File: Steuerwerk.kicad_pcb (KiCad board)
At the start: 2 copper layers, 100 x 160 mm, 115 parts, among them J1 Conn_01x04, J2 Conn_01x02, J3 Conn_01x03, J4 Conn_01x03, J5 Conn_01x02, J6 Conn_01x04, J7 Conn_01x02, J8 Conn_01x04, Q1 Q_PNP_BCE, U1 74LS161, U2 74LS138, U3 74LS138, U4 74240, U5 74LS374, U6 74LS374, U7 74541, U8 74541

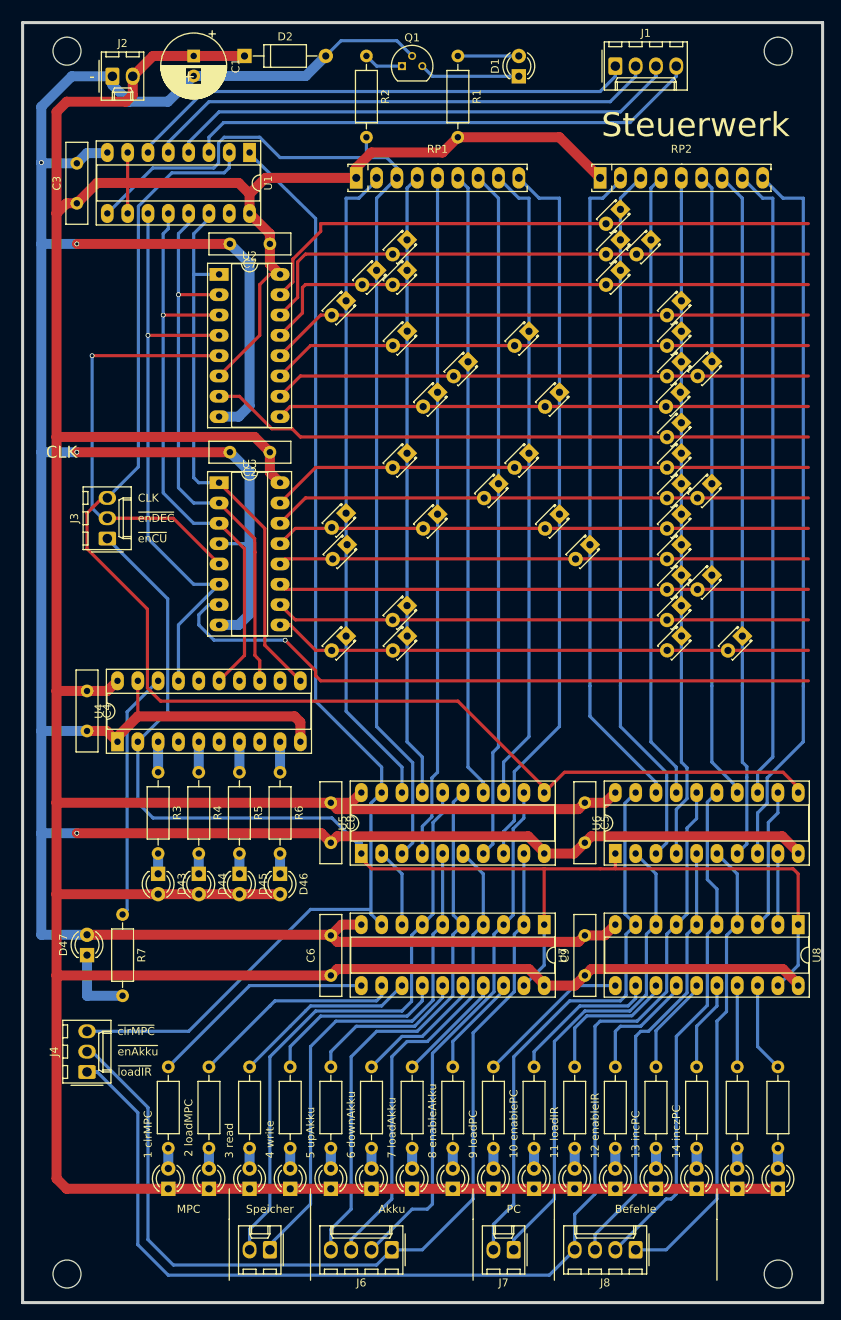
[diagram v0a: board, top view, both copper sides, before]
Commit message: viele Kleinigkeiten
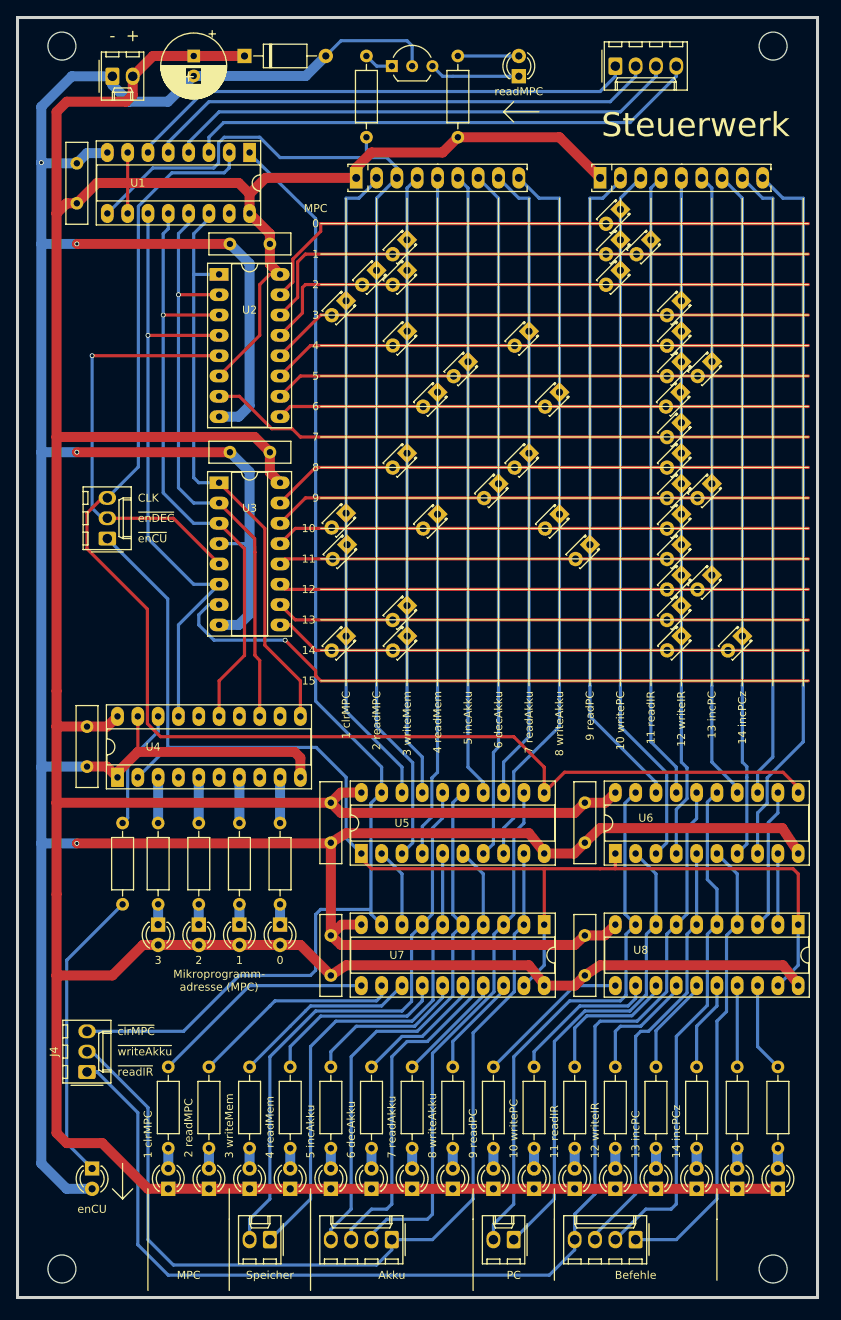
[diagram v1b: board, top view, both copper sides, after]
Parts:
- D2: footprint Diodes_ThroughHole:D_A-405_P10.16mm_Horizontal -> Diode_THT:D_A-405_P10.16mm_Horizontal
- Q1: footprint TO_SOT_Packages_THT:TO-92_Molded_Narrow -> Package_TO_SOT_THT:TO-92_Inline_Wide
- RP1, RP2: footprint Housings_SIP:SIP9_Housing_BigPads -> Package_SIP:SIP9_Housing_BigPads
- U1, U2, U3: footprint Housings_DIP:DIP-16_W7.62mm_Socket_LongPads -> Package_DIP:DIP-16_W7.62mm_Socket_LongPads
- U5: footprint Housings_DIP:DIP-20_W7.62mm_Socket_LongPads -> Package_DIP:DIP-20_W7.62mm_Socket_LongPads
- U6: footprint tg_foodprint:DIP-20_W7.62mm_Socket_LongPadstg -> Package_DIP:DIP-20_W7.62mm_Socket_LongPads
- moved D47 26.7 mm to (49.6, 176.5), turned to 270 degrees
- moved R7 11.4 mm to (53.4, 133.3)
- moved RP1 10.2 mm to (82.6, 52.7)
- moved RP2 10.2 mm to (113.1, 52.7)
- moved R3 6.35 mm to (57.8, 133.3)
- moved R4 6.35 mm to (62.9, 133.3)
- moved R5 6.35 mm to (68.0, 133.3)
- moved R6 6.35 mm to (73.1, 133.3)
- moved D43 6.35 mm to (57.8, 146.0)
- moved D44 6.35 mm to (62.9, 146.0)
- moved D45 6.35 mm to (68.0, 146.0)
- moved D46 6.35 mm to (73.1, 146.0)
- moved C4 4.44 mm to (48.9, 121.2)
- moved U4 4.44 mm to (52.7, 127.6)
- moved Q1 1.27 mm to (87.0, 38.7)
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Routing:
- net Net-(D47-Pad1): track 9.52 -> 37.2 mm
- net VCC: track 602.6 -> 575.7 mm
- net Net-(R7-Pad1): track 31.1 -> 15.2 mm
- net GND: track 486.2 -> 501.2 mm
- net /Takt: track 171.2 -> 176.0 mm
- net Net-(U1-Pad13): track 70.1 -> 74.5 mm
- net Net-(U1-Pad12): track 73.1 -> 77.5 mm
- net Net-(U1-Pad11): track 75.6 -> 80.0 mm
- net Net-(U1-Pad14): track 69.4 -> 73.8 mm
- net /clrMPC: track 146.1 -> 150.2 mm
- net Net-(J5-Pad2): track 73.5 -> 72.2 mm
- net Net-(R6-Pad1): track 3.81 -> 5.08 mm
- net Net-(R5-Pad1): track 3.81 -> 5.08 mm
- net Net-(R4-Pad1): track 3.81 -> 5.08 mm
- net Net-(R3-Pad1): track 3.81 -> 5.08 mm
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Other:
- board text added: "0"
- board text added: "1"
- board text added: "10"
- board text added: "10 writePC"
- board text added: "11"
- board text added: "11 readIR"
- board text added: "12"
- board text added: "12 writeIR"
- board text added: "13"
- board text added: "14"
- board text added: "14 incPCz"
- board text added: "15"
- board text added: "2"
- board text added: "2 readMPC"
- board text added: "3"
- board text added: "3 writeMem"
- board text added: "4"
- board text added: "4 readMem"
- board text added: "5"
- board text added: "5 incAkku"
- board text added: "6"
- board text added: "6 decAkku"
- board text added: "7"
- board text added: "7 readAkku"
- board text added: "8"
- board text added: "8 writeAkku"
- board text added: "9"
- board text added: "9 readPC"
- board text added: "Mikroprogramm- adresse (MPC)"
- board text added: "enCU"
- board text added: "readMPC"
- board text added: "~readIR"
- board text added: "~writeAkku"
- board text removed: "10 enablePC"
- board text removed: "11 loadIR"
- board text removed: "12 enableIR"
- board text removed: "14 inczPC"
- board text removed: "2 loadMPC"
- board text removed: "3 read"
- board text removed: "4 write"
- board text removed: "5 upAkku"
- board text removed: "6 downAkku"
- board text removed: "7 loadAkku"
- board text removed: "8 enableAkku"
- board text removed: "9 loadPC"
- board text removed: "~enAkku"
- board text removed: "~loadIR"
